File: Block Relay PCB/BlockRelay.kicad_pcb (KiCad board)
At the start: 2 copper layers, 157.5 x 99.1 mm, 102 parts, among them J1 Screw_Terminal_01x16, J2 Conn_02x06_Odd_Even, J3 Conn_02x08_Odd_Even, K1 Relay_DPDT, K2 Relay_DPDT, K3 Relay_DPDT, K4 Relay_DPDT, K5 Relay_DPDT, K6 Relay_DPDT, Q1 2N7000, Q2 2N7000, Q3 2N7000, Q4 2N7000, Q5 2N7000, Q6 2N7000, U1 74HC259, U2 74LS251, U5 L78L05_SOT89

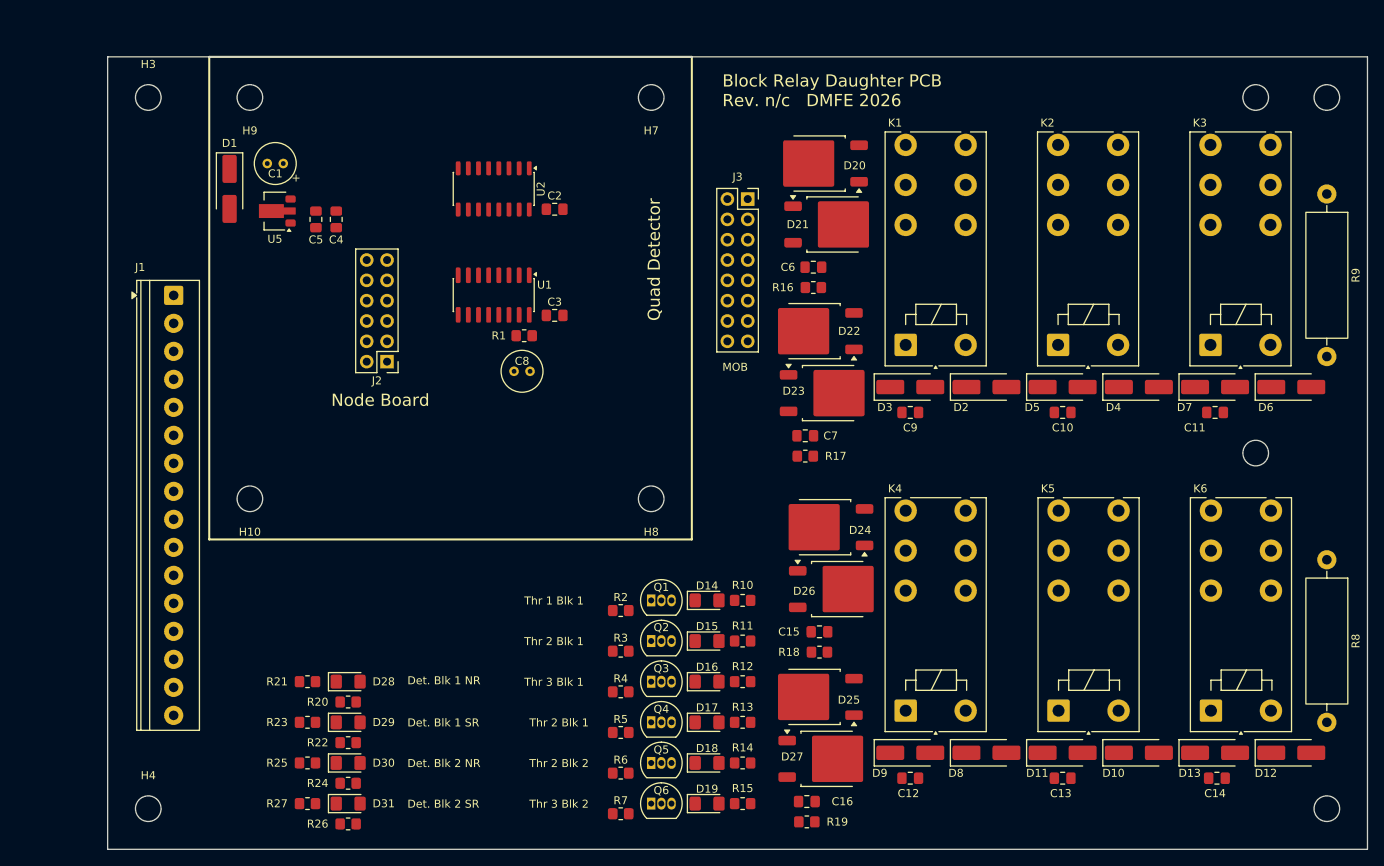
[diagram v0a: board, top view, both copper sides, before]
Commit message: Block Relay ready to print
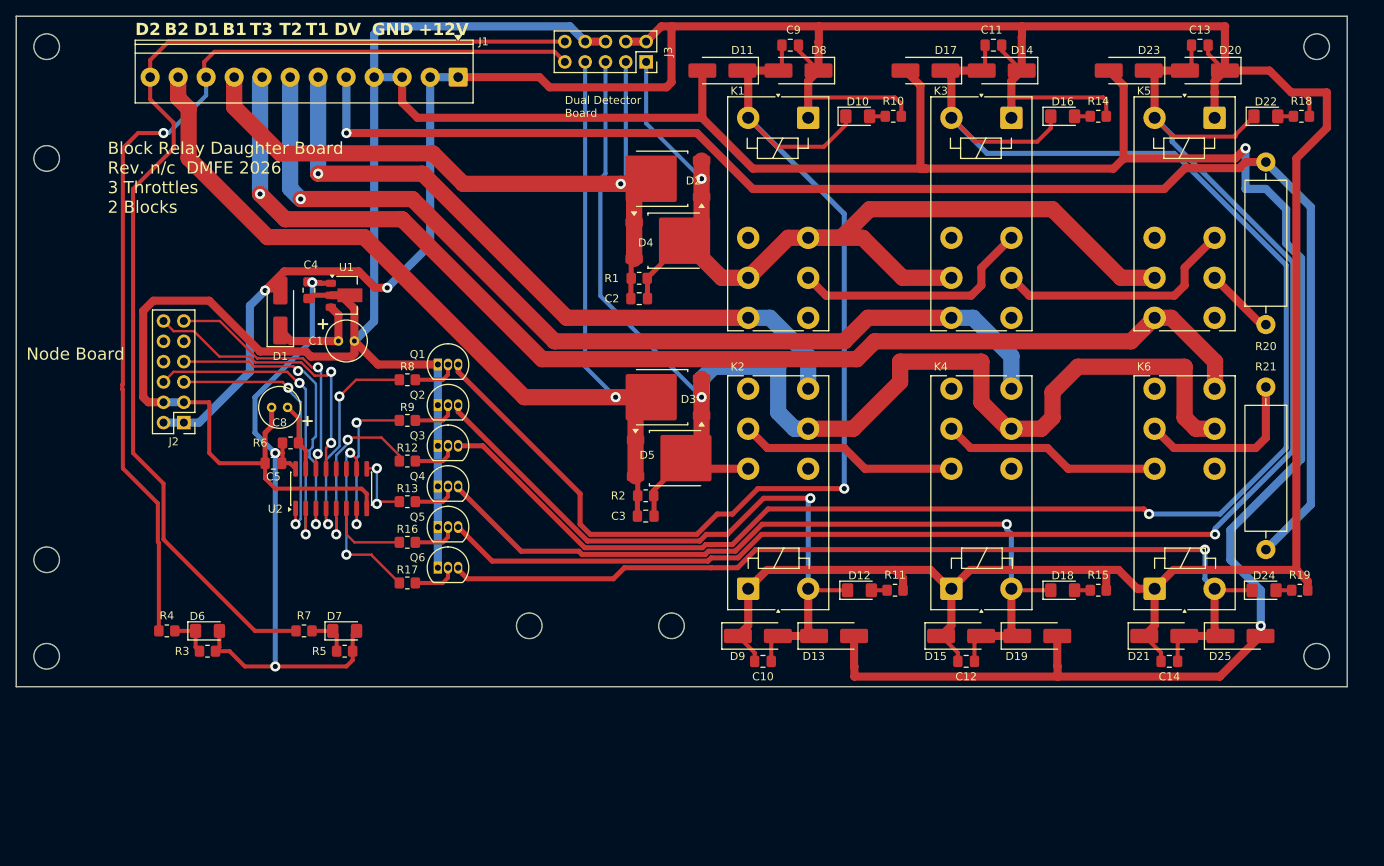
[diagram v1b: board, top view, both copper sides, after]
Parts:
- removed C15, C16, C6, C7: 0.1uF, Capacitor_SMD:C_0805_2012Metric_Pad1.18x1.45mm_HandSolder
- removed D26, D27: Schottky_AKA DPAK, Package_TO_SOT_SMD:TO-252-2
- removed D28, D29, D30, D31: Yellow LED, LED_SMD:LED_1206_3216Metric_Pad1.42x1.75mm_HandSolder
- removed H10, H9: MountingHole, MountingHole:MountingHole_3.2mm_M3
- removed R22, R24, R26: 27K, Resistor_SMD:R_0805_2012Metric_Pad1.20x1.40mm_HandSolder
- removed R23, R25, R27: 2K2, Resistor_SMD:R_0805_2012Metric_Pad1.20x1.40mm_HandSolder
- removed U5: L78L05_SOT89, Package_TO_SOT_SMD:SOT-89-3
- D10, D12, D6, D7: value 1A 1000V -> Yellow LED; footprint Diode_SMD:D_SMA_Handsoldering -> LED_SMD:LED_1206_3216Metric_Pad1.42x1.75mm_HandSolder
- D14, D15, D17, D19: value Yellow LED -> 1A 1000V; footprint LED_SMD:LED_1206_3216Metric_Pad1.42x1.75mm_HandSolder -> Diode_SMD:D_SMA_Handsoldering
- D2, D3, D4, D5: value 1A 1000V -> Schottky_AKA DPAK; footprint Diode_SMD:D_SMA_Handsoldering -> Package_TO_SOT_SMD:TO-252-2
- D20, D21, D23, D25: value Schottky_AKA DPAK -> 1A 1000V; footprint Package_TO_SOT_SMD:TO-252-2 -> Diode_SMD:D_SMA_Handsoldering
- D22, D24: value Schottky_AKA DPAK -> Yellow LED; footprint Package_TO_SOT_SMD:TO-252-2 -> LED_SMD:LED_1206_3216Metric_Pad1.42x1.75mm_HandSolder
- J1: value Screw_Terminal_01x16 -> Screw_Terminal_01x12; footprint TerminalBlock_Phoenix:TerminalBlock_Phoenix_PT-1,5-16-3.5-H_1x16_P3.50mm_Horizontal -> TerminalBlock_Phoenix:TerminalBlock_Phoenix_PT-1,5-12-3.5-H_1x12_P3.50mm_Horizontal
- J3: value Conn_02x08_Odd_Even -> Conn_02x05_Odd_Even; footprint Connector_PinSocket_2.54mm:PinSocket_2x08_P2.54mm_Vertical -> Connector_PinSocket_2.54mm:PinSocket_2x05_P2.54mm_Vertical
- R1: value 4K7 -> 1K0
- R12, R13: value 4K7 -> 47R
- R16, R17: value 1K0 -> 47R
- R18, R19: value 1K0 -> 4K7
- R2: value 47R -> 1K0
- R20: value 27K -> 2K2; footprint Resistor_SMD:R_0805_2012Metric_Pad1.20x1.40mm_HandSolder -> Resistor_THT:R_Axial_DIN0516_L15.5mm_D5.0mm_P20.32mm_Horizontal
- R21: footprint Resistor_SMD:R_0805_2012Metric_Pad1.20x1.40mm_HandSolder -> Resistor_THT:R_Axial_DIN0516_L15.5mm_D5.0mm_P20.32mm_Horizontal
- R3, R5: value 47R -> 27K
- R4, R7: value 47R -> 2K2
- R6: value 47R -> 4K7
- R8, R9: value 2K2 -> 47R; footprint Resistor_THT:R_Axial_DIN0516_L15.5mm_D5.0mm_P20.32mm_Horizontal -> Resistor_SMD:R_0805_2012Metric_Pad1.20x1.40mm_HandSolder
- U1: value 74HC259 -> L78L05_SOT89; footprint Package_SO:SOIC-16_3.9x9.9mm_P1.27mm -> Package_TO_SOT_SMD:SOT-89-3
- U2: value 74LS251 -> 74HC259; footprint Package_SO:SO-16_3.9x9.9mm_P1.27mm -> Package_SO:SOIC-16_3.9x9.9mm_P1.27mm
- moved H6 163.0 mm to (63.5, 89.5), turned to 180 degrees
- moved H5 160.2 mm to (63.5, 39.4), turned to 180 degrees
- moved H2 153.2 mm to (63.5, 101.6)
- moved H1 151.3 mm to (63.5, 25.4)
- moved H4 147.3 mm to (222.2, 101.6)
- moved H3 146.2 mm to (222.2, 25.4)
- moved D6 138.9 mm to (83.6, 98.4)
- moved R21 125.3 mm to (215.9, 67.9), turned to -90 degrees
- moved R20 124.0 mm to (215.9, 60.1), turned to 90 degrees
- moved R9 118.4 mm to (108.6, 72.1), turned to 0 degrees
- moved R8 117.1 mm to (108.6, 67.0), turned to 0 degrees
- moved D7 113.0 mm to (100.7, 98.4)
- moved D11 95.3 mm to (148.0, 28.4), turned to 180 degrees
- moved C13 93.2 mm to (207.6, 25.2), turned to 180 degrees
- moved R14 92.2 mm to (194.9, 34.1)
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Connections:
- C10 pad 2: Net-(D15-K) -> Net-(D12-K)
- C11 pad 2: Net-(D16-K) -> Net-(D14-A)
- C12 pad 2: Net-(D17-K) -> Net-(D15-A)
- C13 pad 2: Net-(D10-K) -> Net-(D20-A)
- C14 pad 2: Net-(D12-K) -> Net-(D21-A)
- C2 pad 1: +5V -> Net-(D2-K)
- C2 pad 2: GND -> Blk1
- C3 pad 1: +5V -> Net-(D3-K)
- C3 pad 2: GND -> Blk2
- C8 pad 1: Net-(U1-Clr) -> Net-(U2-Clr)
- C9 pad 2: Net-(D14-K) -> Net-(D10-K)
- D10 pad 2: GND -> Net-(D10-A)
- D11 pad 1: +12V -> Net-(D10-K)
- D11 pad 2: Net-(D10-K) -> GND
- D12 pad 2: GND -> Net-(D12-A)
- D13 pad 1: +12V -> Net-(D12-K)
- D13 pad 2: Net-(D12-K) -> GND
- D14 pad 1: Net-(D14-K) -> +12V
- D15 pad 1: Net-(D15-K) -> +12V
- D16 pad 1: Net-(D16-K) -> Net-(D14-A)
- D17 pad 1: Net-(D17-K) -> Net-(D14-A)
- D17 pad 2: Net-(D17-A) -> GND
- D18 pad 1: Net-(D10-K) -> Net-(D15-A)
- D19 pad 1: Net-(D12-K) -> Net-(D15-A)
- D19 pad 2: Net-(D19-A) -> GND
- D2 pad 1: Net-(D14-K) -> Blk1
- D2 pad 2: GND -> Net-(D2-K)
- D20 pad 1: Blk1 -> +12V
- D20 pad 2: Net-(D20-K) -> Net-(D20-A)
- D21 pad 1: Net-(D20-K) -> +12V
- D21 pad 2: Blk1 -> Net-(D21-A)
- D22 pad 1: TrkGnd -> Net-(D20-A)
- D22 pad 2: Net-(D22-K) -> Net-(D22-A)
- D23 pad 1: Net-(D22-K) -> Net-(D20-A)
- D23 pad 2: TrkGnd -> GND
- D24 pad 1: Blk2 -> Net-(D21-A)
- D24 pad 2: Net-(D24-K) -> Net-(D24-A)
- D25 pad 1: TrkGnd -> Net-(D21-A)
- D25 pad 2: Net-(D25-K) -> GND
- D3 pad 1: +12V -> Blk2
- D3 pad 2: Net-(D14-K) -> Net-(D3-K)
- D4 pad 1: Net-(D15-K) -> Net-(D2-K)
- D4 pad 2: GND -> Blk1
- D5 pad 1: +12V -> Net-(D3-K)
- D5 pad 2: Net-(D15-K) -> Blk2
- D6 pad 1: Net-(D16-K) -> Net-(D6-K)
- D6 pad 2: GND -> +5V
- D7 pad 1: +12V -> Net-(D7-K)
- D7 pad 2: Net-(D16-K) -> +5V
- D8 pad 1: Net-(D17-K) -> +12V
- D8 pad 2: GND -> Net-(D10-K)
- D9 pad 2: Net-(D17-K) -> Net-(D12-K)
- J1 pad 10: Net-(D20-K) -> Net-(J1-Pin_10)
- J1 pad 11: Net-(D22-K) -> Net-(D3-K)
- J1 pad 12: Net-(D24-K) -> Net-(J1-Pin_12)
- J1 pad 5: TrkGnd -> Det12V
- J1 pad 6: Det12V -> Thr1
- J1 pad 7: Thr1 -> Thr2
- J1 pad 8: Thr2 -> Thr3
- J1 pad 9: Thr3 -> Net-(D2-K)
- J2 pad 10: nE1 -> unconnected-(J2-Pin_10-Pad10)
- J2 pad 11: nE2 -> nE
- J2 pad 8: A3 -> unconnected-(J2-Pin_8-Pad8)
- J2 pad 9: A4 -> unconnected-(J2-Pin_9-Pad9)
- J3 pad 10: Net-(J3-Pin_10) -> Net-(J1-Pin_12)
- J3 pad 3: Net-(D20-K) -> Net-(D2-K)
- J3 pad 5: TrkGnd -> Blk2
- J3 pad 7: Net-(D22-K) -> Net-(D3-K)
- J3 pad 9: Blk2 -> Net-(J1-Pin_10)
- K1 pad A2: Net-(D14-K) -> Net-(D10-K)
- K2 pad 12: Net-(K1-Pad11) -> Blk2
- K2 pad 21: Blk1 -> Blk2
- K2 pad 24: Thr2 -> Thr1
- K2 pad A2: Net-(D15-K) -> Net-(D12-K)
- K3 pad 12: Net-(K2-Pad11) -> Net-(K1-Pad11)
- K3 pad 24: Thr3 -> Thr2
- K3 pad A2: Net-(D16-K) -> Net-(D14-A)
- K4 pad 12: Blk2 -> Net-(K2-Pad11)
- K4 pad 24: Thr1 -> Thr2
- K4 pad A2: Net-(D17-K) -> Net-(D15-A)
- K5 pad 12: Net-(K4-Pad11) -> Net-(K3-Pad11)
- K5 pad 21: Blk2 -> Blk1
- K5 pad 24: Thr2 -> Thr3
- K5 pad A2: Net-(D10-K) -> Net-(D20-A)
- K6 pad 12: Net-(K5-Pad11) -> Net-(K4-Pad11)
- K6 pad A2: Net-(D12-K) -> Net-(D21-A)
- Q1 pad 3: Net-(D14-K) -> Net-(D10-K)
- Q2 pad 3: Net-(D15-K) -> Net-(D12-K)
- Q3 pad 3: Net-(D16-K) -> Net-(D14-A)
- Q4 pad 3: Net-(D17-K) -> Net-(D15-A)
- Q5 pad 3: Net-(D10-K) -> Net-(D20-A)
- Q6 pad 3: Net-(D12-K) -> Net-(D21-A)
- R1 pad 1: +5V -> Net-(D2-K)
- R1 pad 2: Net-(U1-Clr) -> Blk1
- R10 pad 2: Net-(D14-A) -> Net-(D10-A)
- R11 pad 2: Net-(D15-A) -> Net-(D12-A)
- R12 pad 1: +12V -> Net-(U2-Q1)
- R12 pad 2: Net-(D16-A) -> Net-(Q3-G)
- R13 pad 1: +12V -> Net-(U2-Q4)
- R13 pad 2: Net-(D17-A) -> Net-(Q4-G)
- R14 pad 2: Net-(D18-A) -> Net-(D16-A)
- R15 pad 2: Net-(D19-A) -> Net-(D18-A)
- R16 pad 1: Net-(D20-K) -> Net-(U2-Q2)
- R16 pad 2: Blk1 -> Net-(Q5-G)
- R17 pad 1: Net-(D22-K) -> Net-(U2-Q5)
- R17 pad 2: TrkGnd -> Net-(Q6-G)
- R18 pad 1: Net-(D24-K) -> +12V
- R18 pad 2: Blk2 -> Net-(D22-A)
- R19 pad 1: Net-(D25-K) -> +12V
- R19 pad 2: TrkGnd -> Net-(D24-A)
- R2 pad 1: Net-(U1-Q0) -> Net-(D3-K)
- R2 pad 2: Net-(Q1-G) -> Blk2
- R20 pad 1: +5V -> Net-(K5-Pad11)
- R20 pad 2: Net-(D28-K) -> Det12V
- R21 pad 1: Net-(D28-K) -> Net-(K6-Pad11)
- R21 pad 2: Net-(J3-Pin_10) -> Det12V
- R3 pad 1: Net-(U1-Q1) -> +5V
- R3 pad 2: Net-(Q2-G) -> Net-(D6-K)
- R4 pad 1: Net-(U1-Q2) -> Net-(D6-K)
- R4 pad 2: Net-(Q3-G) -> Net-(J1-Pin_10)
- R5 pad 1: Net-(U1-Q3) -> +5V
- R5 pad 2: Net-(Q4-G) -> Net-(D7-K)
- R6 pad 1: Net-(U1-Q4) -> +5V
- R6 pad 2: Net-(Q5-G) -> Net-(U2-Clr)
- R7 pad 1: Net-(U1-Q5) -> Net-(D7-K)
- R7 pad 2: Net-(Q6-G) -> Net-(J1-Pin_12)
- R8 pad 1: Net-(K6-Pad11) -> Net-(U2-Q0)
- R8 pad 2: Det12V -> Net-(Q1-G)
- R9 pad 1: Net-(K3-Pad11) -> Net-(U2-Q3)
- R9 pad 2: Det12V -> Net-(Q2-G)
- U1 pad 1: A0 -> +5V
- U1 pad 2: A1 -> GND
- U1 pad 3: A2 -> Net-(D1-K)
- U2 pad 1: Net-(J3-Pin_16) -> A0
- U2 pad 10: A1 -> Net-(U2-Q5)
- U2 pad 11: A0 -> unconnected-(U2-Q6-Pad11)
- U2 pad 13: unconnected-(U2-I6-Pad13) -> Data
- U2 pad 14: unconnected-(U2-I5-Pad14) -> nE
- U2 pad 15: unconnected-(U2-I4-Pad15) -> Net-(U2-Clr)
- U2 pad 2: Net-(J3-Pin_14) -> A1
- U2 pad 3: Net-(J3-Pin_12) -> A2
- U2 pad 4: Net-(J3-Pin_10) -> Net-(U2-Q0)
- U2 pad 5: Data -> Net-(U2-Q1)
- U2 pad 6: unconnected-(U2-~{Y}-Pad6) -> Net-(U2-Q2)
- U2 pad 7: nE2 -> Net-(U2-Q3)
- U2 pad 9: A2 -> Net-(U2-Q4)
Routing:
- net GND: track 0.00 -> 487.9 mm, vias 0 -> 2
- net +12V: track 0.00 -> 453.7 mm, vias 0 -> 2
- net Net-(D14-A): track 0.00 -> 216.7 mm, vias 0 -> 1
- net Net-(D20-A): track 0.00 -> 189.8 mm, vias 0 -> 1
- net Det12V: track 0.00 -> 179.3 mm, vias 0 -> 1
- net Blk2: track 0.00 -> 172.4 mm, vias 0 -> 1
- net Thr3: track 0.00 -> 150.5 mm, vias 0 -> 1
- net Net-(D3-K): track 0.00 -> 144.6 mm, vias 0 -> 1
- net Net-(D10-K): track 0.00 -> 143.5 mm, vias 0 -> 1
- net Net-(J1-Pin_12): track 0.00 -> 138.9 mm
- net Net-(J1-Pin_10): track 0.00 -> 125.8 mm, vias 0 -> 1
- net Blk1: track 0.00 -> 125.3 mm, vias 0 -> 1
- net Net-(D21-A): track 0.00 -> 120.0 mm, vias 0 -> 1
- net Thr2: track 0.00 -> 119.3 mm, vias 0 -> 1
- net Net-(D15-A): track 0.00 -> 101.3 mm, vias 0 -> 1
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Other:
- board size 157.5 x 99.1 mm -> 166.4 x 83.8 mm
- board text added: "+12V"
- board text added: "B1"
- board text added: "B2"
- board text added: "Block Relay Daughter Board Rev. n/c DMFE 2026 3 Throttles 2 Blocks"
- board text added: "D1"
- board text added: "D2"
- board text added: "DV"
- board text added: "Dual Detector Board"
- board text added: "GND"
- board text added: "T1"
- board text added: "T2"
- board text added: "T3"
- board text removed: "Block Relay Daughter PCB Rev. n/c DMFE 2026"
- board text removed: "Det. Blk 1 NR"
- board text removed: "Det. Blk 1 SR"
- board text removed: "Det. Blk 2 NR"
- board text removed: "Det. Blk 2 SR"
- board text removed: "MOB"
- board text removed: "Quad Detector"
- board text removed: "Thr 1 Blk 1"
- board text removed: "Thr 2 Blk 1"
- board text removed: "Thr 2 Blk 2"
- board text removed: "Thr 3 Blk 1"
- board text removed: "Thr 3 Blk 2"
